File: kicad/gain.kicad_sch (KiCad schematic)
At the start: 10 parts, among them U7 TCA9548APWR

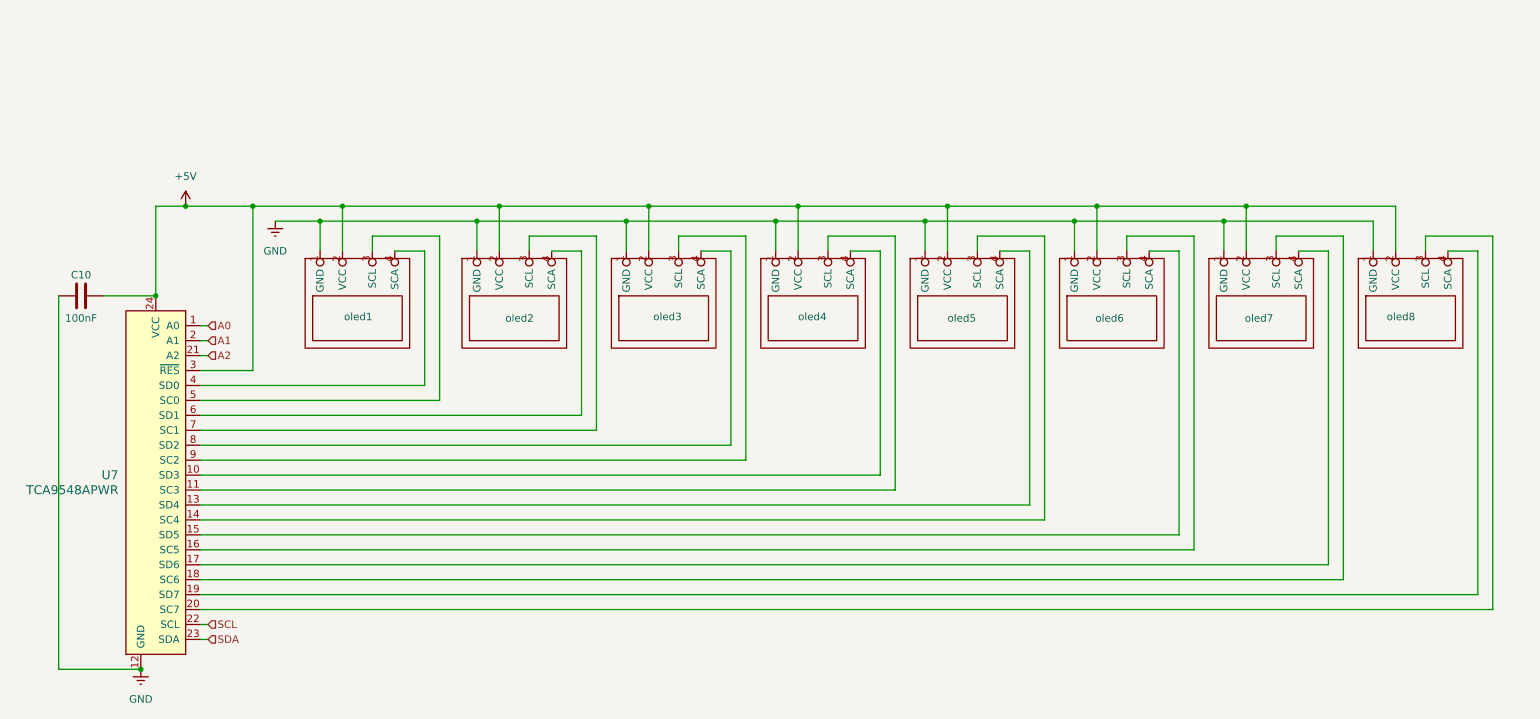
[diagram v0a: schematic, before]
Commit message: kicad updates
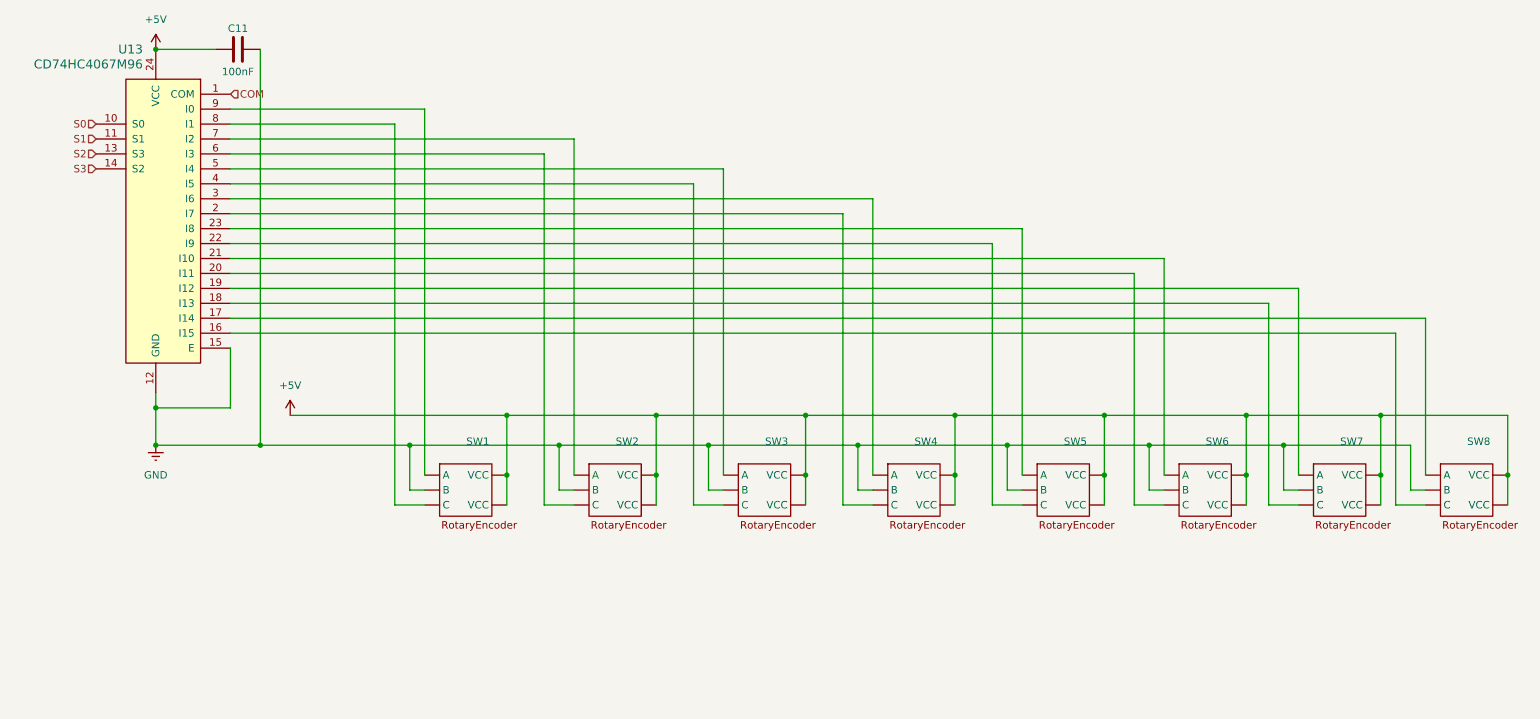
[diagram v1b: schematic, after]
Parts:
- removed C10: 100nF, Capacitor_THT:C_Axial_L5.1mm_D3.1mm_P7.50mm_Horizontal, symbol Device:C
- removed U7: TCA9548APWR, digikey-footprints:TSSOP-24_W4.40mm, symbol dk_Logic-Signal-Switches-Multiplexers-Decoders:TCA9548APWR
- removed oled1, oled2, oled3, oled4, oled5, oled6, oled7, oled8: ~, mixer:oled, symbol mixer:ssd1306
- added C11: 100nF, Capacitor_THT:C_Axial_L5.1mm_D3.1mm_P7.50mm_Horizontal, symbol Device:C
- added SW1, SW2, SW3, SW4, SW5, SW6, SW7, SW8: ~, mixer:RotaryEncoder, symbol mixer:rotary_encoder
- added U13: CD74HC4067M96, digikey-footprints:SOIC-24_W7.50mm, symbol dk_Interface-Analog-Switches-Multiplexers-Demultiplexers:CD74HC4067M96
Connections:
- net +5V: now also C11.1, SW1. (VCC), SW2. (VCC), SW3. (VCC), SW4. (VCC), SW5. (VCC), SW6. (VCC), SW7. (VCC), SW8. (VCC), U13.24 (VCC)
- net GND: now also C11.2, SW1. (VCC), SW2. (VCC), SW3. (VCC), SW4. (VCC), SW5. (VCC), SW6. (VCC), SW7. (VCC), SW8. (VCC), U13.12 (GND), U13.15 (E)
- new net: SW5. (VCC), U13.22 (I9)
- new net: SW5. (VCC), U13.23 (I8)
- new net: SW2. (VCC), U13.6 (I3)
- new net: SW2. (VCC), U13.7 (I2)
- new net: SW1. (VCC), U13.8 (I1)
- new net: SW1. (VCC), U13.9 (I0)
- new net: SW7. (VCC), U13.18 (I13)
- new net: SW7. (VCC), U13.19 (I12)
- new net: SW8. (VCC), U13.16 (I15)
- new net: SW8. (VCC), U13.17 (I14)
- new net: SW3. (VCC), U13.4 (I5)
- new net: SW3. (VCC), U13.5 (I4)
- new net: SW4. (VCC), U13.2 (I7)
- new net: SW6. (VCC), U13.20 (I11)
- new net: SW6. (VCC), U13.21 (I10)
- new net: SW4. (VCC), U13.3 (I6)
- new net COM: U13.1 (COM)
- new net S0: U13.10 (S0)
- new net S1: U13.11 (S1)
- new net S2: U13.13 (S3)
- new net S3: U13.14 (S2)

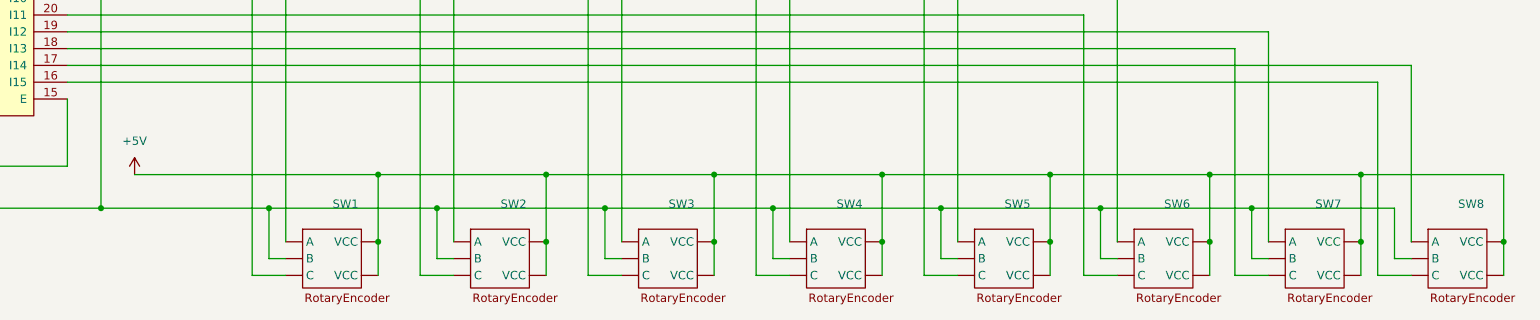
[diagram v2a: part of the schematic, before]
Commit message: pcb routing 2
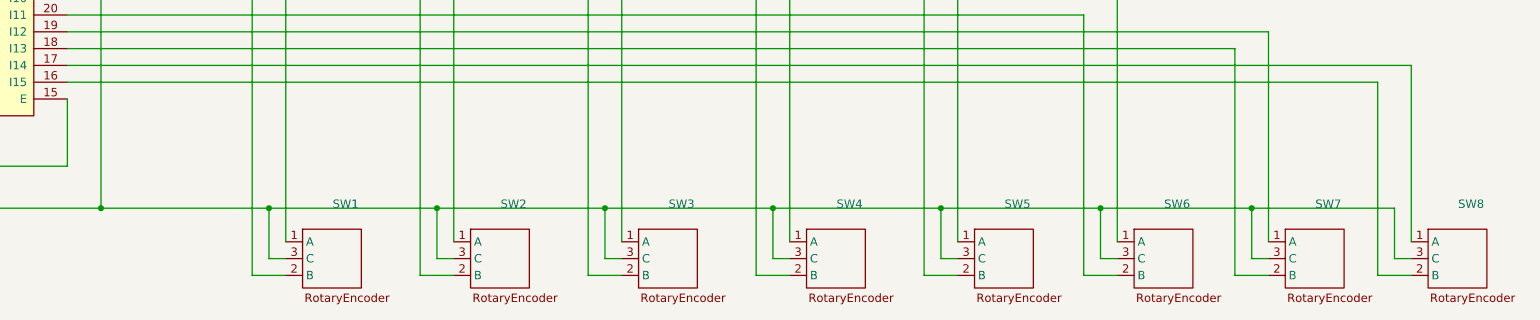
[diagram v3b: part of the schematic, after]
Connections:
- net +5V: no longer SW1. (VCC), SW2. (VCC), SW3. (VCC), SW4. (VCC), SW5. (VCC), SW6. (VCC), SW7. (VCC), SW8. (VCC)
- net GND: now also SW1.3 (C), SW2.3 (C), SW3.3 (C), SW4.3 (C), SW5.3 (C), SW6.3 (C), SW7.3 (C), SW8.3 (C); no longer SW1. (VCC), SW2. (VCC), SW3. (VCC), SW4. (VCC), SW5. (VCC), SW6. (VCC), SW7. (VCC), SW8. (VCC)
- net at U13.22 (I9): now also SW5.2 (B); no longer SW5. (VCC)
- net at U13.23 (I8): now also SW5.1 (A); no longer SW5. (VCC)
- net at U13.6 (I3): now also SW2.2 (B); no longer SW2. (VCC)
- net at U13.7 (I2): now also SW2.1 (A); no longer SW2. (VCC)
- net at U13.8 (I1): now also SW1.2 (B); no longer SW1. (VCC)
- net at U13.9 (I0): now also SW1.1 (A); no longer SW1. (VCC)
- net at U13.18 (I13): now also SW7.2 (B); no longer SW7. (VCC)
- net at U13.19 (I12): now also SW7.1 (A); no longer SW7. (VCC)
- net at U13.16 (I15): now also SW8.2 (B); no longer SW8. (VCC)
- net at U13.17 (I14): now also SW8.1 (A); no longer SW8. (VCC)
- net at U13.4 (I5): now also SW3.2 (B); no longer SW3. (VCC)
- net at U13.5 (I4): now also SW3.1 (A); no longer SW3. (VCC)
- net at U13.2 (I7): now also SW4.2 (B); no longer SW4. (VCC)
- net at U13.20 (I11): now also SW6.2 (B); no longer SW6. (VCC)
- net at U13.21 (I10): now also SW6.1 (A); no longer SW6. (VCC)
- net at U13.3 (I6): now also SW4.1 (A); no longer SW4. (VCC)
